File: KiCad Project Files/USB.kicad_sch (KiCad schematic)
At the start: 6 parts, among them J1 SM04B, U3 XC6206PxxxMR, U4 PRTR5V0U2X

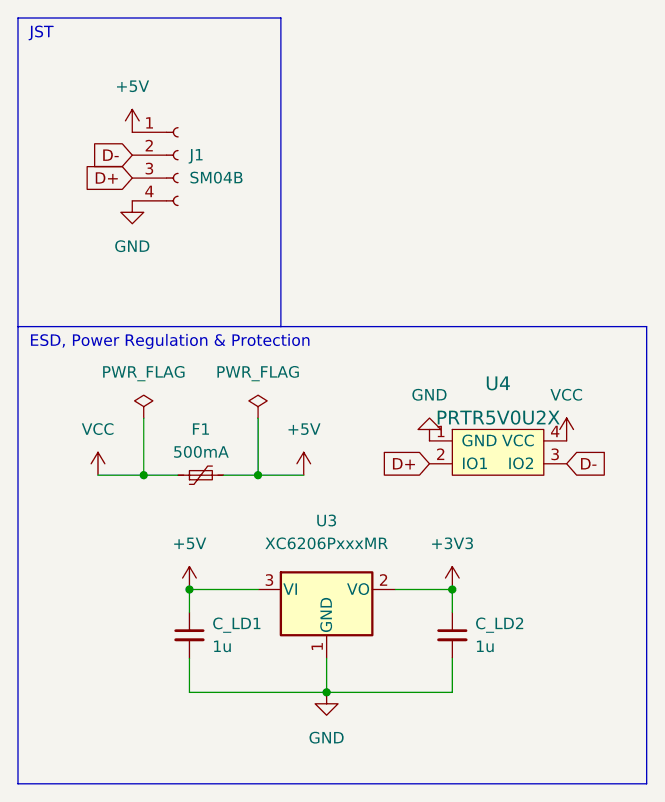
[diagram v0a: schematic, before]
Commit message: Finish PCB and create production files
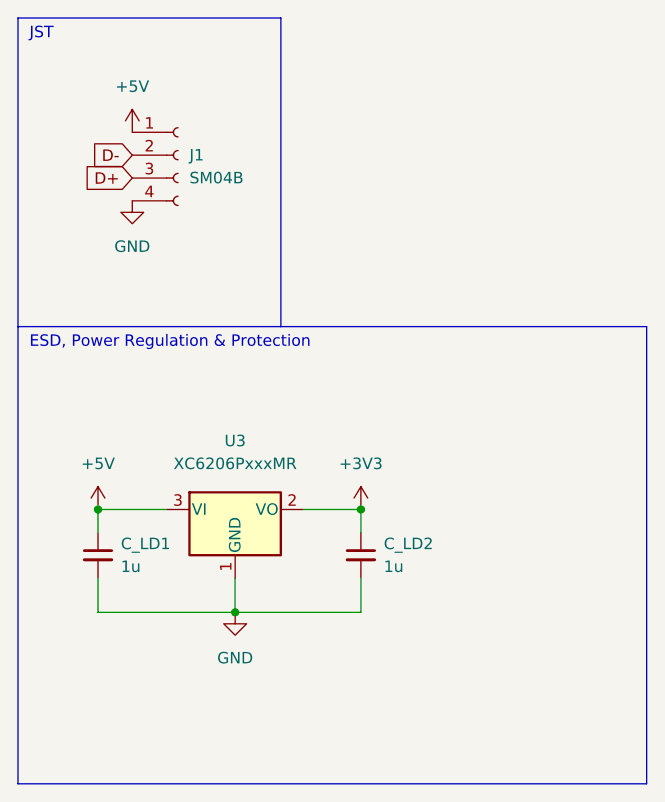
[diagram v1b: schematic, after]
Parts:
- removed F1: 500mA, Fuse:Fuse_0805_2012Metric, symbol Device:Polyfuse_Small
- removed U4: PRTR5V0U2X, random-keyboard-parts:SOT143B, symbol cipulot_parts:PRTR5V0U2X
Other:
- moved on the sheet: C_LD1, C_LD2, U3
